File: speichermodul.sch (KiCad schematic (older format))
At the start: 64 parts, among them IC1 6116, P1 CONN_3X2, P2 CONN_01X01, P3 CONN_01X01, P4 CONN_01X01, P5 CONN_01X01, P6 CONN_01X01, P7 CONN_01X01, P8 CONN_02X10, P9 CONN_02X10, SW1 SW_PUSH, SW2 SW_PUSH, U1 7400, U2 74LS08, U3 74LS08, U4 74LS14, U5 74LS540, U6 74LS540

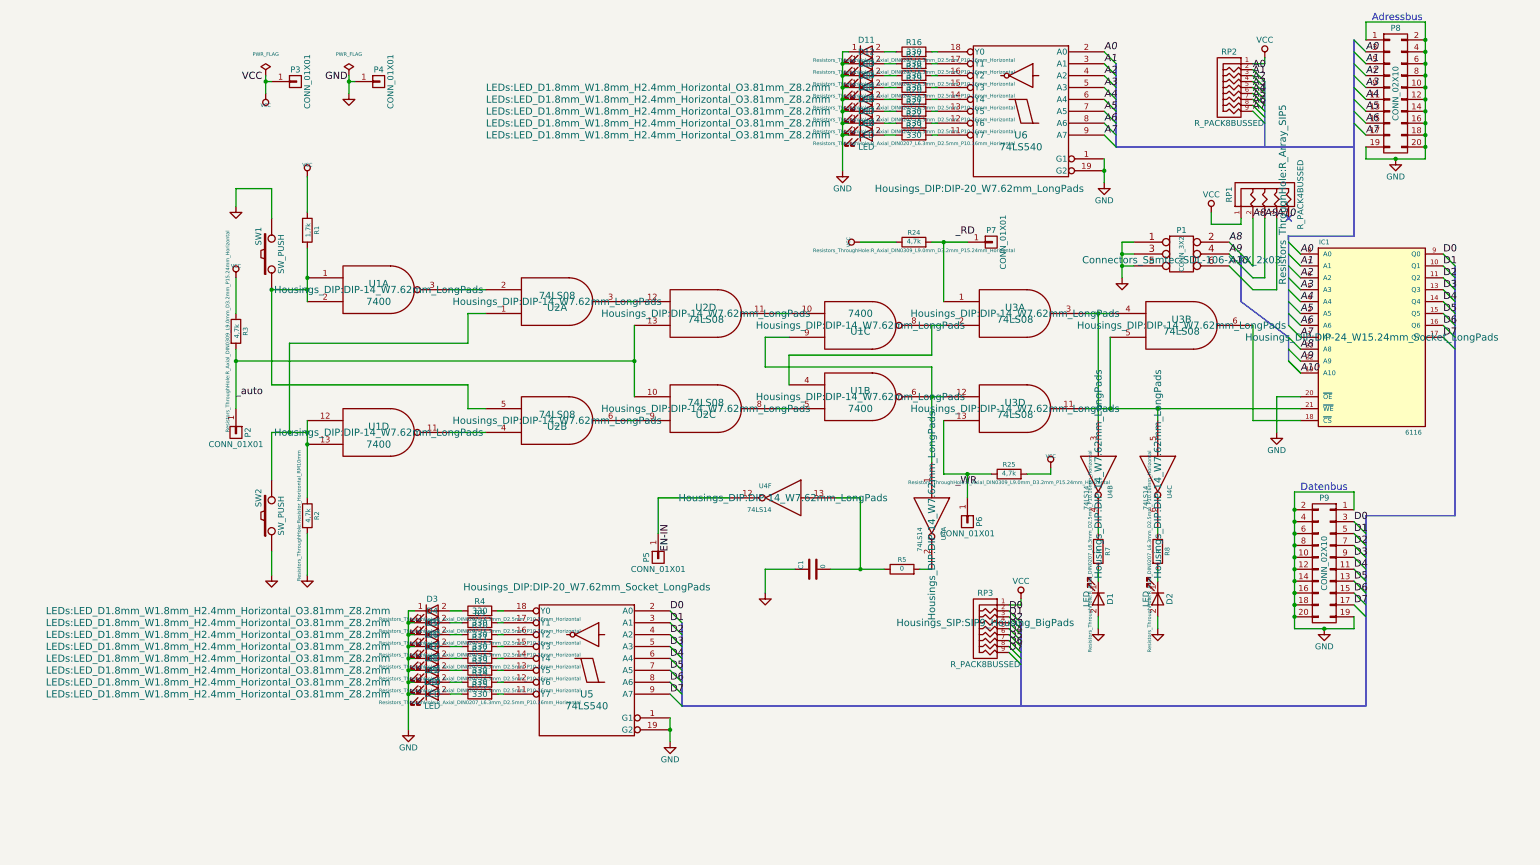
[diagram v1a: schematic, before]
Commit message: Pcb layout kabelverlegt
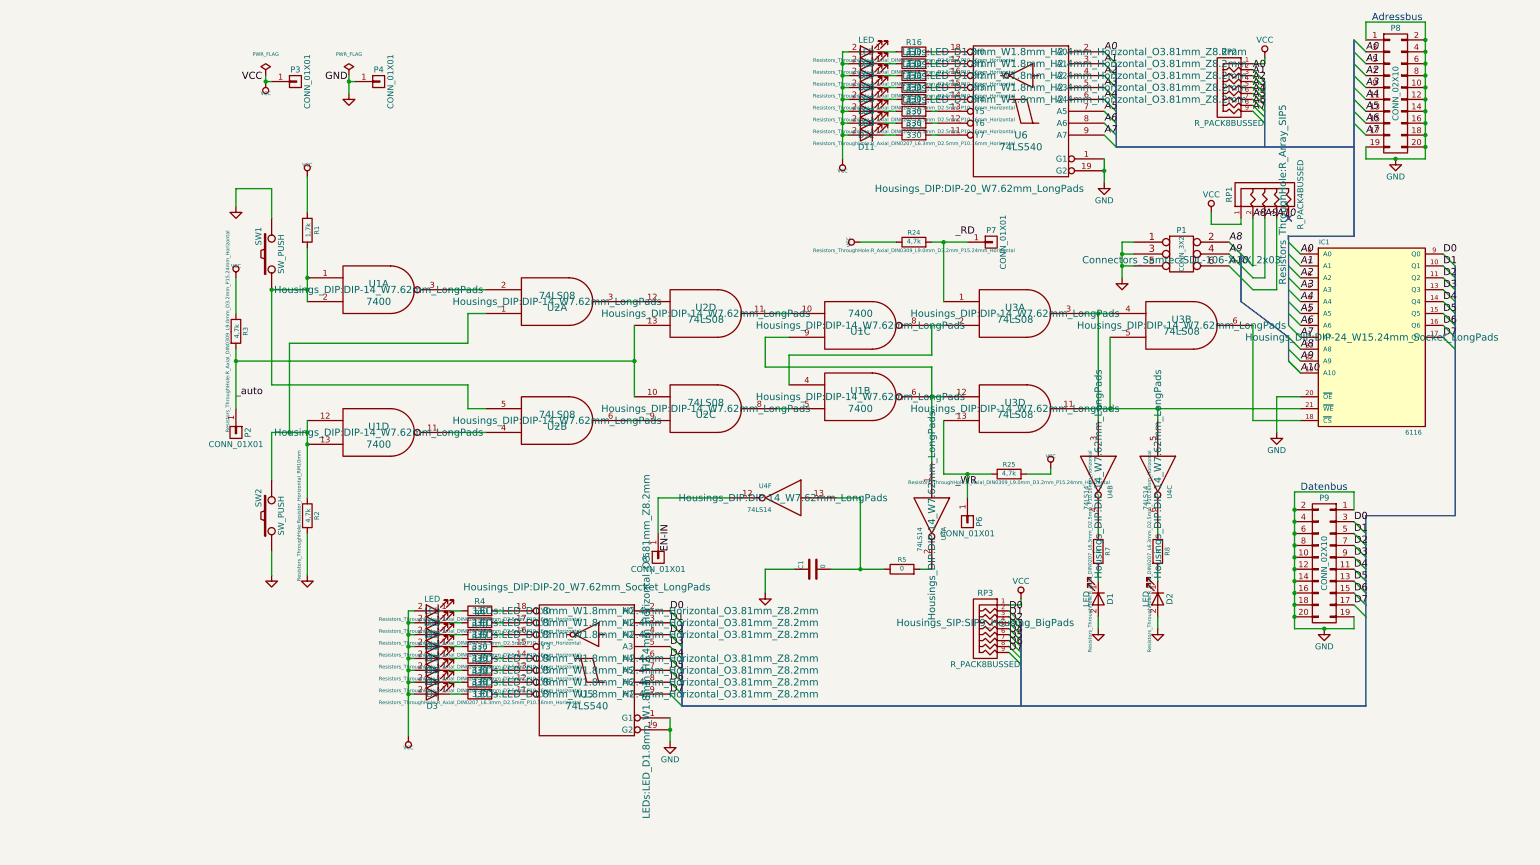
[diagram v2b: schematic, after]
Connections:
- net GND: no longer D10.1 (K), D11.1 (K), D12.1 (K), D13.1 (K), D14.1 (K), D15.1 (K), D16.1 (K), D17.1 (K), D18.1 (K), D3.1 (K), D4.1 (K), D5.1 (K), D6.1 (K), D7.1 (K), D8.1 (K), D9.1 (K)
- net VCC: now also D10.2 (A), D11.2 (A), D12.2 (A), D13.2 (A), D14.2 (A), D15.2 (A), D16.2 (A), D17.2 (A), D18.2 (A), D3.2 (A), D4.2 (A), D5.2 (A), D6.2 (A), D7.2 (A), D8.2 (A), D9.2 (A)
- net at R4.1: now also D10.1 (K); no longer D3.2 (A)
- net at R9.1: now also D9.1 (K); no longer D4.2 (A)
- net at R10.1: now also D8.1 (K); no longer D5.2 (A)
- net at R11.1: now also D7.1 (K); no longer D6.2 (A)
- net at R12.1: now also D6.1 (K); no longer D7.2 (A)
- net at R13.1: now also D5.1 (K); no longer D8.2 (A)
- net at R14.1: now also D4.1 (K); no longer D9.2 (A)
- net at R15.1: now also D3.1 (K); no longer D10.2 (A)
- net at R16.1: now also D18.1 (K); no longer D11.2 (A)
- net at R17.1: now also D17.1 (K); no longer D12.2 (A)
- net at R18.1: now also D16.1 (K); no longer D13.2 (A)
- net at R19.1: now also D15.1 (K); no longer D14.2 (A)
- net at R20.1: now also D14.1 (K); no longer D15.2 (A)
- net at R21.1: now also D13.1 (K); no longer D16.2 (A)
- net at R22.1: now also D12.1 (K); no longer D17.2 (A)
- net at R23.1: now also D11.1 (K); no longer D18.2 (A)
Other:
- moved on the sheet: D10, D11, D12, D13, D14, D15, D16, D17, D18, D3, D4, D5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
